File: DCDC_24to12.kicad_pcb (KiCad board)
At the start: 2 copper layers, 61.6 x 36.7 mm, 28 parts, among them J1 Power_IN, J2 Power_OUT, U1 BD9F800MUX-ZE2

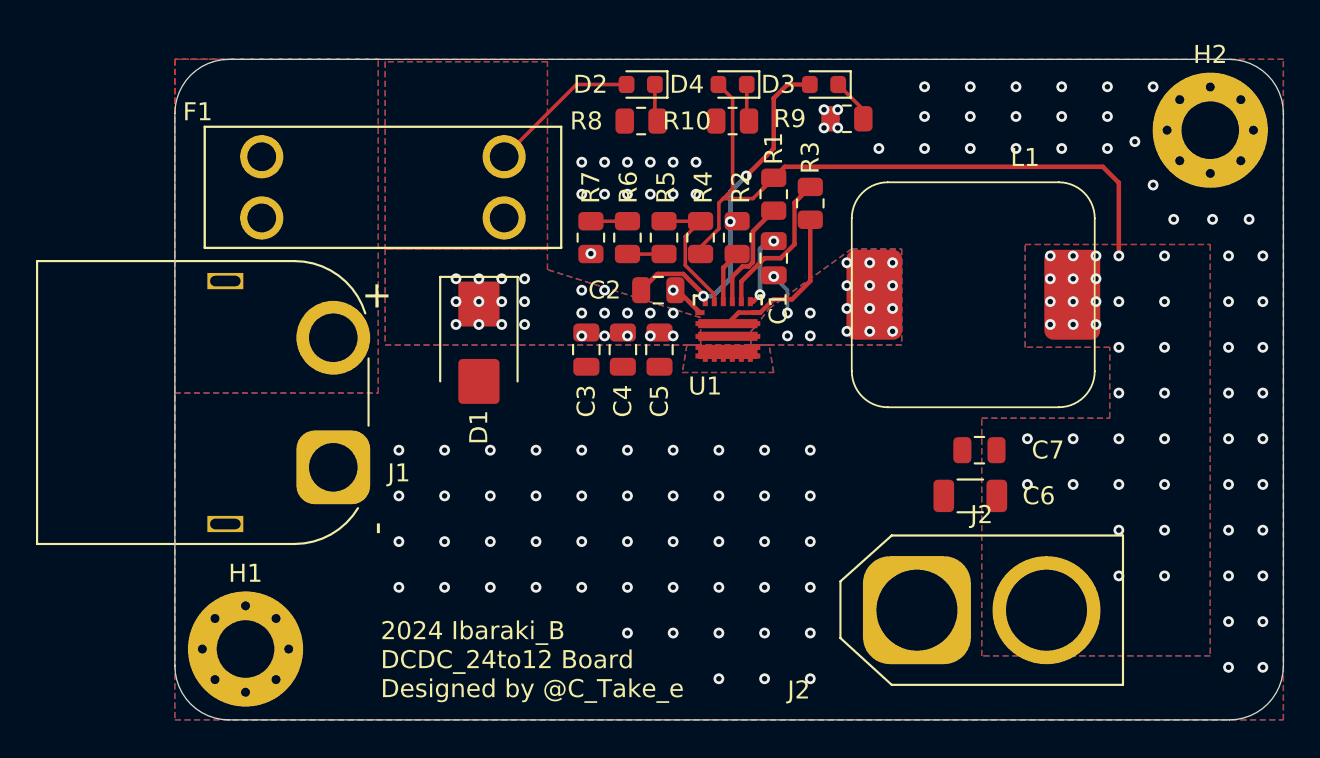
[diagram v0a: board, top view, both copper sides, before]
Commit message: だいぶ小型化
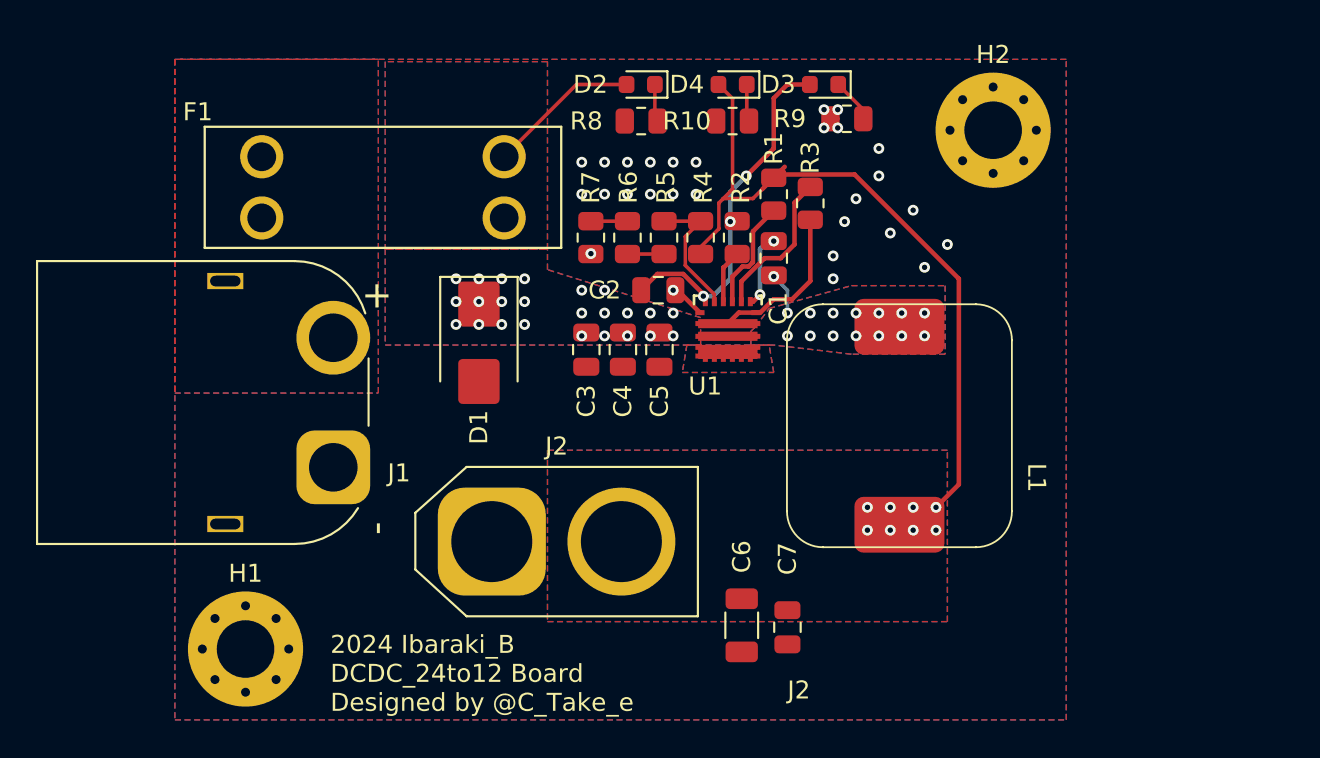
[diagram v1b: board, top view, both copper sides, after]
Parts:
- moved J2 23.9 mm to (89.0, 66.0)
- moved C6 14.6 mm to (102.9, 70.7), turned to -90 degrees
- moved C7 14.5 mm to (105.4, 70.8), turned to -90 degrees
- moved H2 12.1 mm to (116.8, 43.2)
- moved L1 2.26 mm to (111.6, 54.1), turned to -90 degrees
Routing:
- net +12V: track 37.5 -> 40.5 mm, vias 32 -> 8
- net SW: vias 17 -> 15
- net GND: vias 108 -> 28
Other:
- board outline removed
